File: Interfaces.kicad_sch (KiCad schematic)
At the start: 2 parts, among them J5 Conn_01x05_Pin, J6 Conn_01x05_Pin

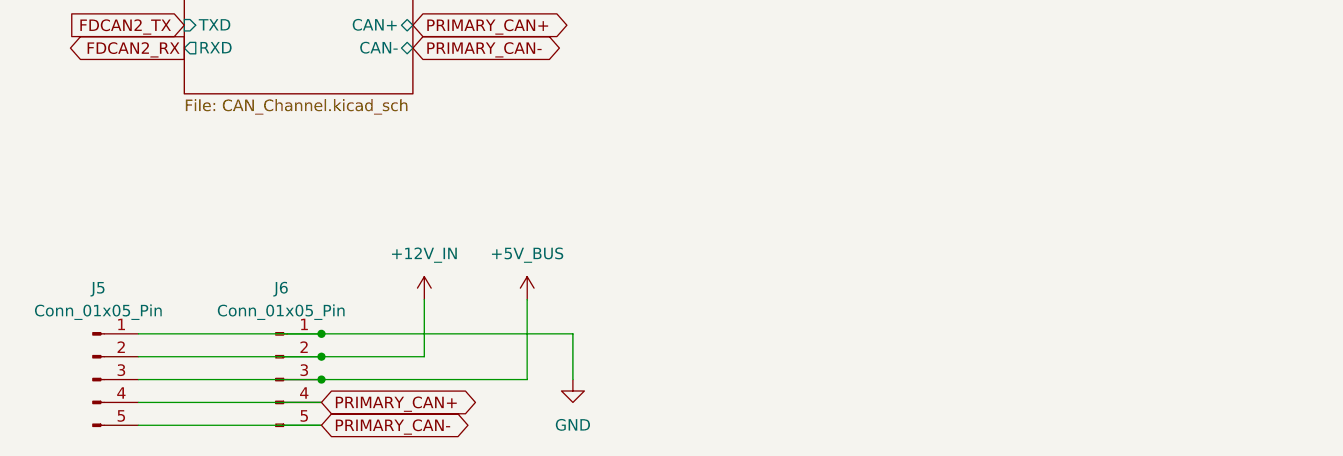
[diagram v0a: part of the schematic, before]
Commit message: LCD connector, backlight, other work
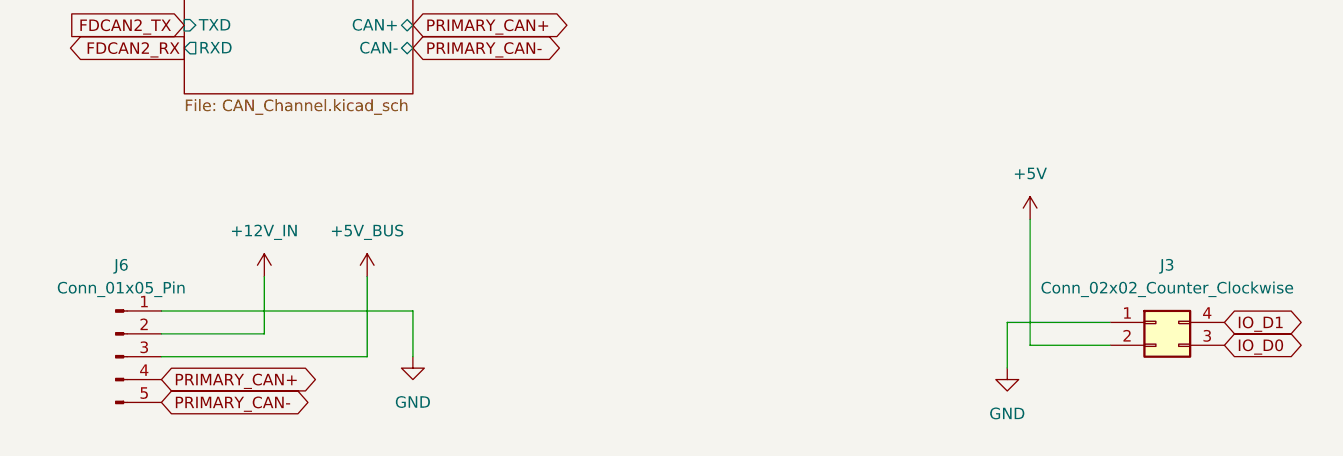
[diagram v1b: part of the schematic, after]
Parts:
- removed J5: Conn_01x05_Pin, Connector_Molex:Molex_Micro-Fit_3.0_43650-0515_1x05_P3.00mm_Vertical, symbol Connector:Conn_01x05_Pin
- added J3: Conn_02x02_Counter_Clockwise, Connector_Molex:Molex_Micro-Fit_3.0_43045-0412_2x02_P3.00mm_Vertical, symbol Connector_Generic:Conn_02x02_Counter_Clockwise
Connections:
- net GND: now also J3.1 (Pin_1)
- new net +5V: J3.2 (Pin_2)
- new net IO_D0: J3.3 (Pin_3)
- new net IO_D1: J3.4 (Pin_4)
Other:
- moved on the sheet: J6

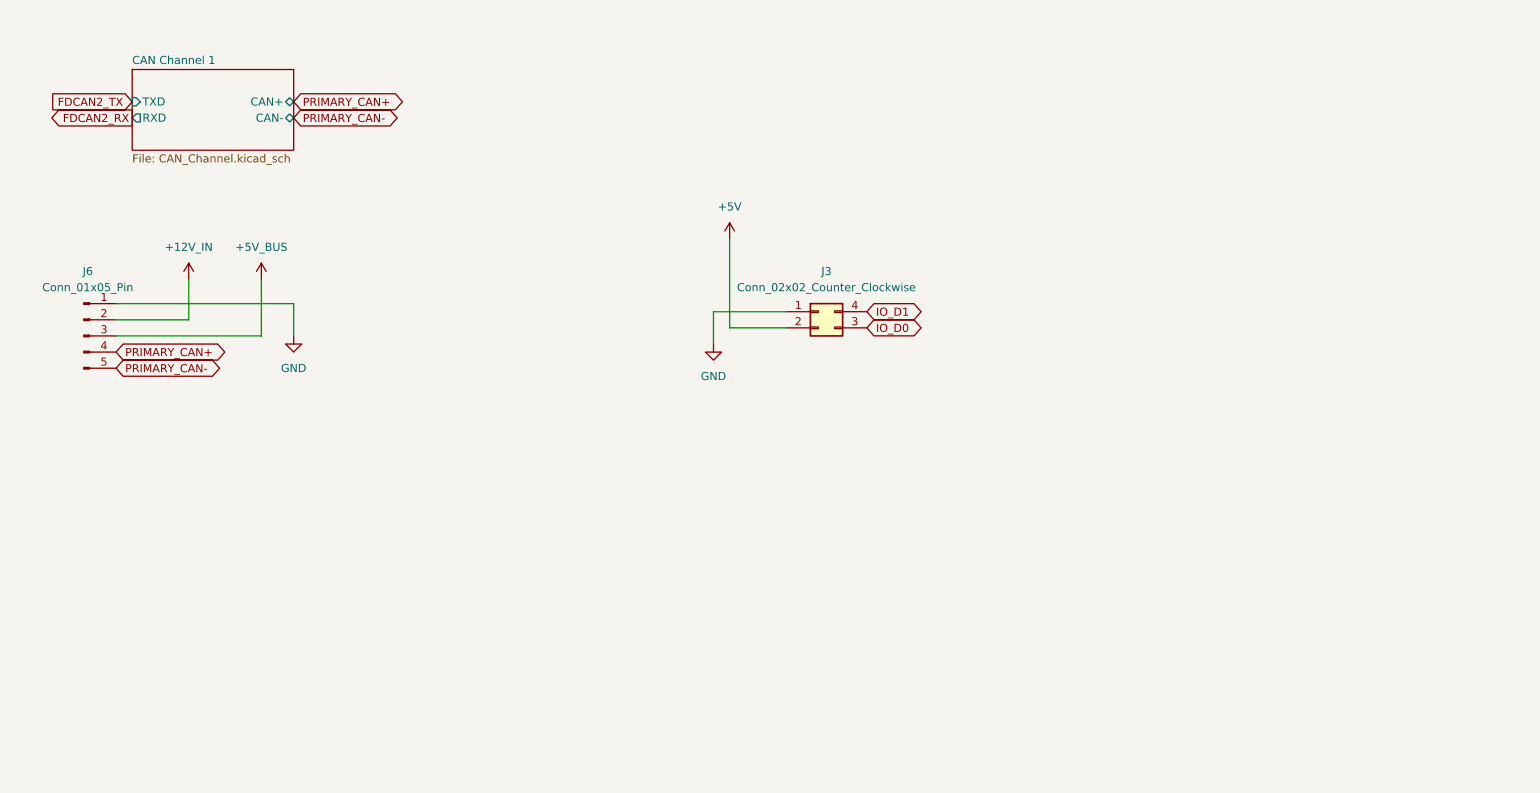
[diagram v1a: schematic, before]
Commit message: preliminary complete schematic
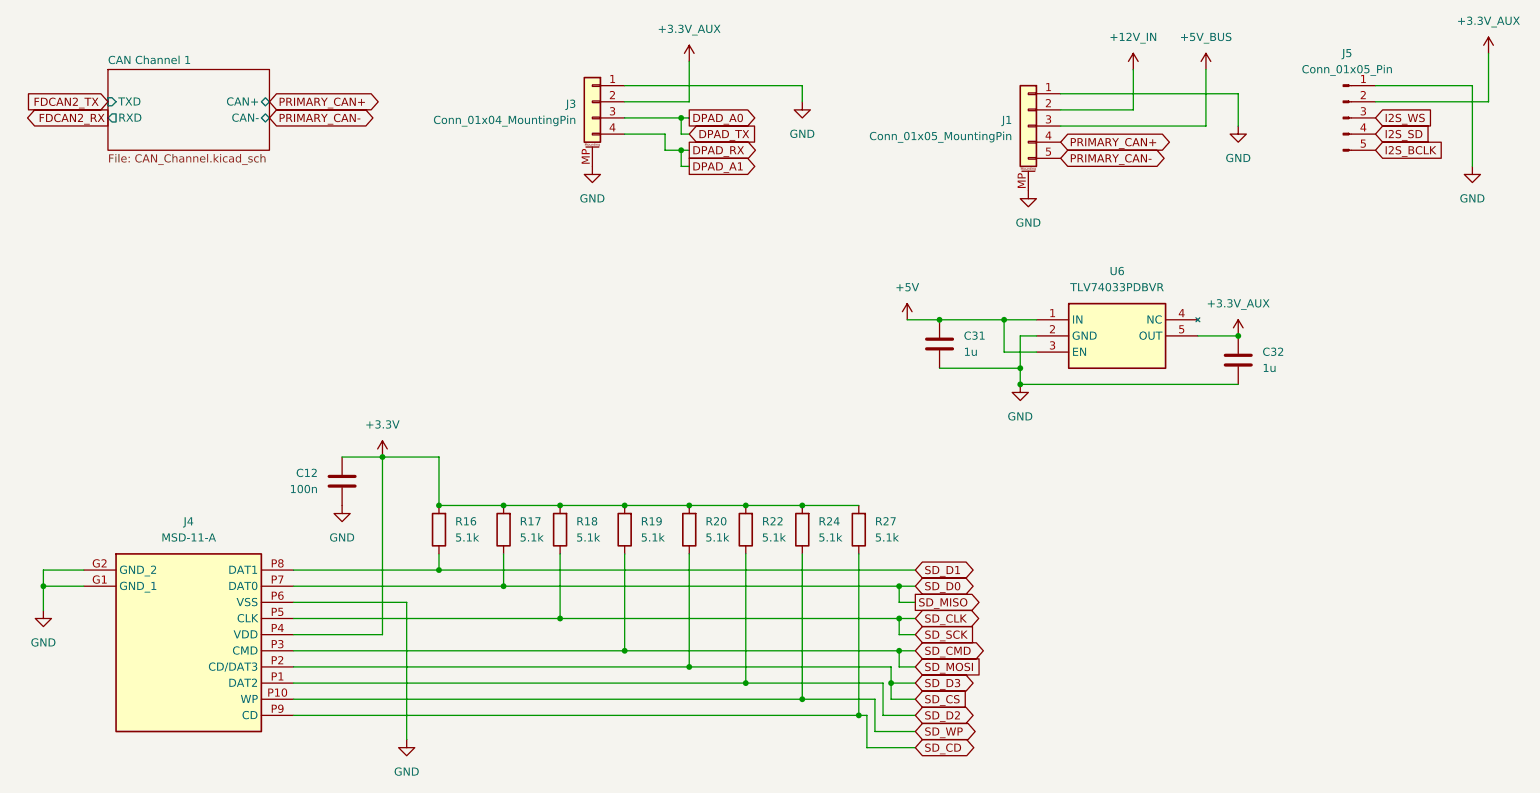
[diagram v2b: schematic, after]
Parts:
- removed J3: Conn_02x02_Counter_Clockwise, Connector_Molex:Molex_Micro-Fit_3.0_43045-0412_2x02_P3.00mm_Vertical, symbol Connector_Generic:Conn_02x02_Counter_Clockwise
- removed J6: Conn_01x05_Pin, Connector_Molex:Molex_Micro-Fit_3.0_43650-0515_1x05_P3.00mm_Vertical, symbol Connector:Conn_01x05_Pin
- added C12: 100n, Capacitor_SMD:C_0603_1608Metric_Pad1.08x0.95mm_HandSolder, symbol Device:C
- added C31, C32: 1u, Capacitor_SMD:C_0603_1608Metric_Pad1.08x0.95mm_HandSolder, symbol Device:C
- added J1: Conn_01x05_MountingPin, Connector_Molex:Molex_Micro-Fit_3.0_43650-0510_1x05-1MP_P3.00mm_Horizontal, symbol Connector_Generic_MountingPin:Conn_01x05_MountingPin
- added J3: Conn_01x04_MountingPin, Connector_Molex:Molex_Micro-Fit_3.0_43650-0410_1x04-1MP_P3.00mm_Horizontal, symbol Connector_Generic_MountingPin:Conn_01x04_MountingPin
- added J4: MSD-11-A, SamacSys_Parts:MSD11A, symbol SamacSys_Parts:MSD-11-A
- added J5: Conn_01x05_Pin, Connector_PinHeader_2.54mm:PinHeader_1x05_P2.54mm_Vertical, symbol Connector:Conn_01x05_Pin
- added R16, R17, R18, R19, R20, R22, R24, R27: 5.1k, Resistor_SMD:R_0603_1608Metric_Pad0.98x0.95mm_HandSolder, symbol Device:R
- added U6: TLV74033PDBVR, SamacSys_Parts:SOT95P280X145-5N, symbol SamacSys_Parts:TLV74033PDBVR
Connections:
- net +12V_IN: now also J1.2 (Pin_2)
- net +5V: now also C31.1, U6.1 (IN), U6.3 (EN)
- net +5V_BUS: now also J1.3 (Pin_3)
- net GND: now also C12.2, C31.2, C32.2, J1.1 (Pin_1), J1.MP (MountPin), J3.1 (Pin_1), J3.MP (MountPin), J4.G1 (GND_1), J4.G2 (GND_2), J4.P6 (VSS), J5.1 (Pin_1), U6.2 (GND)
- net PRIMARY_CAN+: now also J1.4 (Pin_4)
- net PRIMARY_CAN-: now also J1.5 (Pin_5)
- new net +3.3V: C12.1, J4.P4 (VDD), R16.2, R17.2, R18.2, R19.2, R20.2, R22.2, R24.2, R27.2
- new net +3.3V_AUX: C32.1, J3.2 (Pin_2), J5.2 (Pin_2), U6.5 (OUT)
- new net DPAD_A0: J3.3 (Pin_3)
- new net DPAD_A1: J3.4 (Pin_4)
- new net I2S_BCLK: J5.5 (Pin_5)
- new net I2S_SD: J5.4 (Pin_4)
- new net I2S_WS: J5.3 (Pin_3)
- new net SD_CD: J4.P9 (CD), R27.1
- new net SD_CLK: J4.P5 (CLK), R18.1
- new net SD_CMD: J4.P3 (CMD), R19.1
- new net SD_CS: J4.P2 (CD/DAT3), R20.1
- new net SD_D0: J4.P7 (DAT0), R17.1
- new net SD_D1: J4.P8 (DAT1), R16.1
- new net SD_D2: J4.P1 (DAT2), R22.1
- new net SD_WP: J4.P10 (WP), R24.1
